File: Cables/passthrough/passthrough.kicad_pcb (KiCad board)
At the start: 2 copper layers, 40 x 18.5 mm, 32 parts, among them J1 DB25_Male, J10 Conn_01x01, J11 Conn_01x01, J12 Conn_01x01, J13 Conn_01x01, J14 Conn_01x01, J15 Conn_01x01, J16 Conn_01x01, J17 Conn_01x01, J18 Conn_01x01, J19 Conn_01x01, J2 Conn_01x01, J20 Conn_01x01, J21 Conn_01x01, J22 Conn_01x01, J23 Conn_01x01, J24 Conn_01x01, J25 Conn_01x01, J26 Conn_01x01, J27 Conn_01x01, J28 Conn_01x01, J29 Conn_01x01, J3 Conn_01x01, J30 Conn_01x01, J31 Conn_01x01, J4 Conn_01x01, J5 Conn_01x01, J6 Conn_01x01, J7 Conn_01x01, J8 Conn_01x01, J9 Conn_01x01

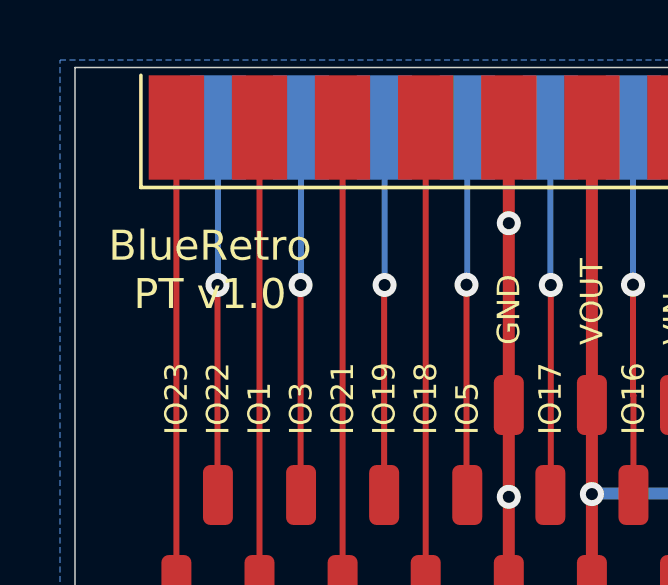
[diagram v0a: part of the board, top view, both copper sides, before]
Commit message: Tweak PT & LS PCBs
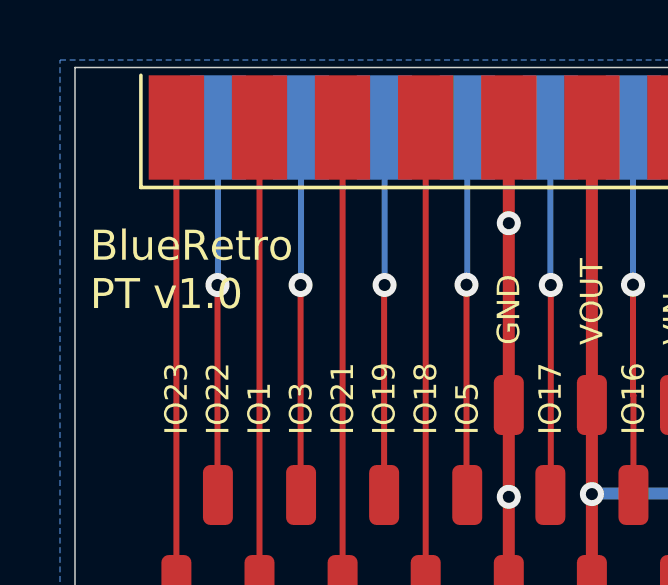
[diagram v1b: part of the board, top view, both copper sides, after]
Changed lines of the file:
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@@
   )
   (page A4)
+  (title_block
+    (title "BlueRetro Passthrough cable adapter")
+    (date 2020-09-05)
+    (rev v1.0)
+  )
   (layers
     (0 F.Cu signal)
@@
     (effects (font (size 1 1) (thickness 0.15)) (justify left mirror))
   )
-  (gr_text "BlueRetro\nPT v1.0" (at -15.5 -2.5) (layer F.SilkS)
-    (effects (font (size 1 1) (thickness 0.15)))
+  (gr_text "BlueRetro\nPT v1.0" (at -19.5 -2.5) (layer F.SilkS)
+    (effects (font (size 1 1) (thickness 0.15)) (justify left))
   )
   (gr_text LO (at 4.99 -4.12) (layer F.SilkS)
